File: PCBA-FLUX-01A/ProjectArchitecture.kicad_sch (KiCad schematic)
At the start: 0 parts

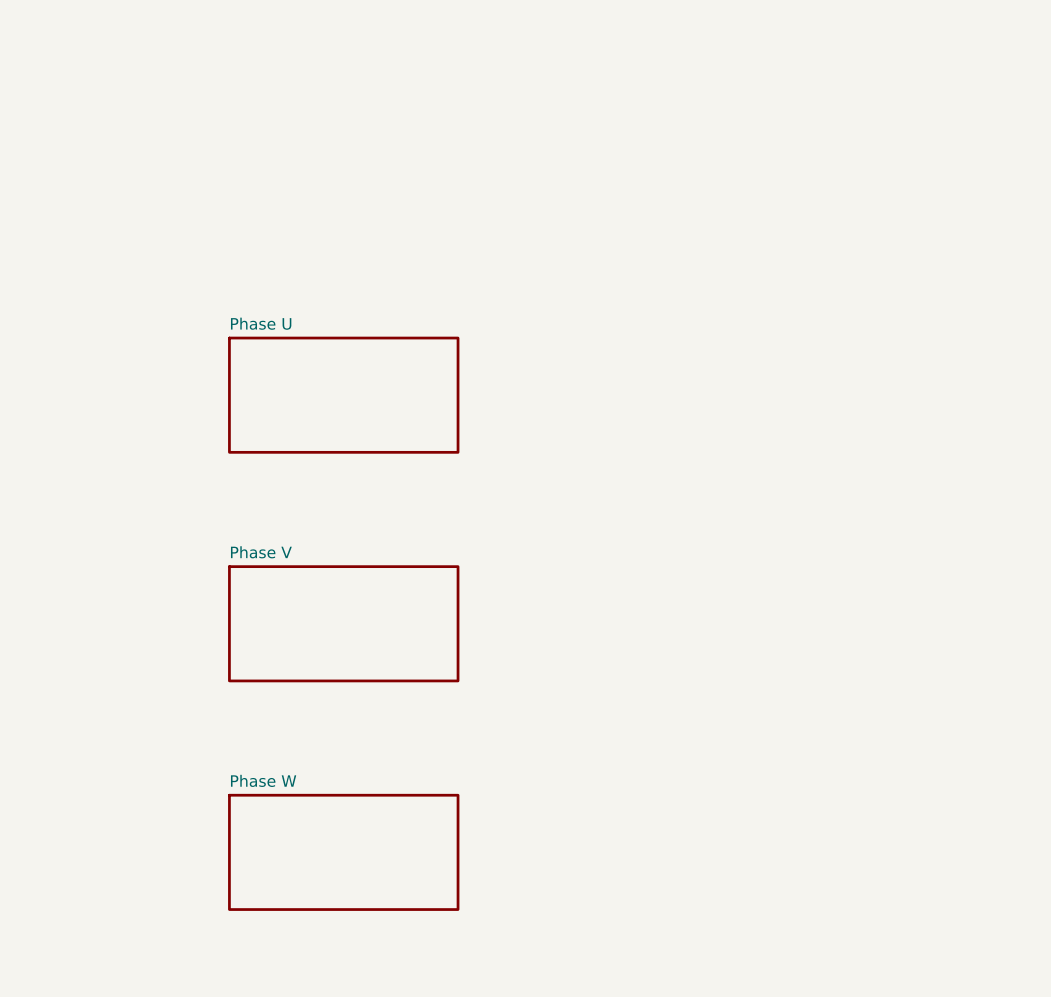
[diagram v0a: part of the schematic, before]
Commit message: Changes were made
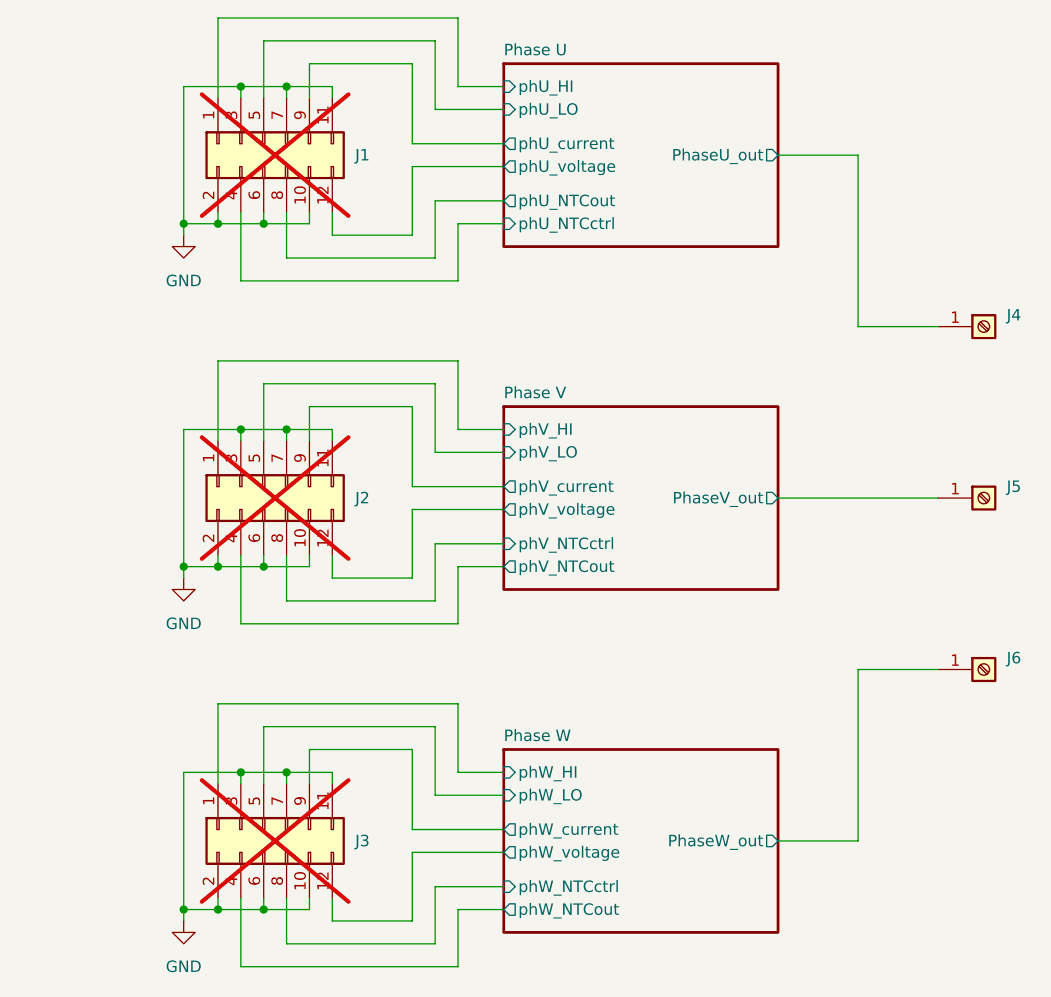
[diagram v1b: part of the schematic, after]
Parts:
- added J1, J2, J3: Conn_02x06_Odd_Even, Connector_PinHeader_2.54mm:PinHeader_2x06_P2.54mm_Vertical, symbol Connector_Generic:Conn_02x06_Odd_Even
- added J4, J5, J6: Screw_Terminal_01x01, symbol Connector:Screw_Terminal_01x01
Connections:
- new net GND: J1.10 (Pin_10), J1.11 (Pin_11), J1.2 (Pin_2), J1.3 (Pin_3), J1.6 (Pin_6), J1.7 (Pin_7), J2.10 (Pin_10), J2.11 (Pin_11), J2.2 (Pin_2), J2.3 (Pin_3), J2.6 (Pin_6), J2.7 (Pin_7), J3.10 (Pin_10), J3.11 (Pin_11), J3.2 (Pin_2), J3.3 (Pin_3), J3.6 (Pin_6), J3.7 (Pin_7)
- new net Phase U/PhaseU_out: J4.1 (Pin_1)
- new net Phase U/phU_HI: J1.1 (Pin_1)
- new net Phase U/phU_LO: J1.5 (Pin_5)
- new net Phase U/phU_NTCctrl: J1.4 (Pin_4)
- new net Phase U/phU_NTCout: J1.8 (Pin_8)
- new net Phase U/phU_current: J1.9 (Pin_9)
- new net Phase U/phU_voltage: J1.12 (Pin_12)
- new net Phase V/PhaseV_out: J5.1 (Pin_1)
- new net Phase V/phV_HI: J2.1 (Pin_1)
- new net Phase V/phV_LO: J2.5 (Pin_5)
- new net Phase V/phV_NTCctrl: J2.8 (Pin_8)
- new net Phase V/phV_NTCout: J2.4 (Pin_4)
- new net Phase V/phV_current: J2.9 (Pin_9)
- new net Phase V/phV_voltage: J2.12 (Pin_12)
- new net Phase W/PhaseW_out: J6.1 (Pin_1)
- new net Phase W/phW_HI: J3.1 (Pin_1)
- new net Phase W/phW_LO: J3.5 (Pin_5)
- new net Phase W/phW_NTCctrl: J3.8 (Pin_8)
- new net Phase W/phW_NTCout: J3.4 (Pin_4)
- new net Phase W/phW_current: J3.9 (Pin_9)
- new net Phase W/phW_voltage: J3.12 (Pin_12)
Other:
- sheet Phase U ports: added PhaseU_out, phU_HI, phU_LO, phU_NTCctrl, phU_NTCout, phU_current, phU_voltage; removed none
- sheet Phase V ports: added PhaseV_out, phV_HI, phV_LO, phV_NTCctrl, phV_NTCout, phV_current, phV_voltage; removed none
- sheet Phase W ports: added PhaseW_out, phW_HI, phW_LO, phW_NTCctrl, phW_NTCout, phW_current, phW_voltage; removed none

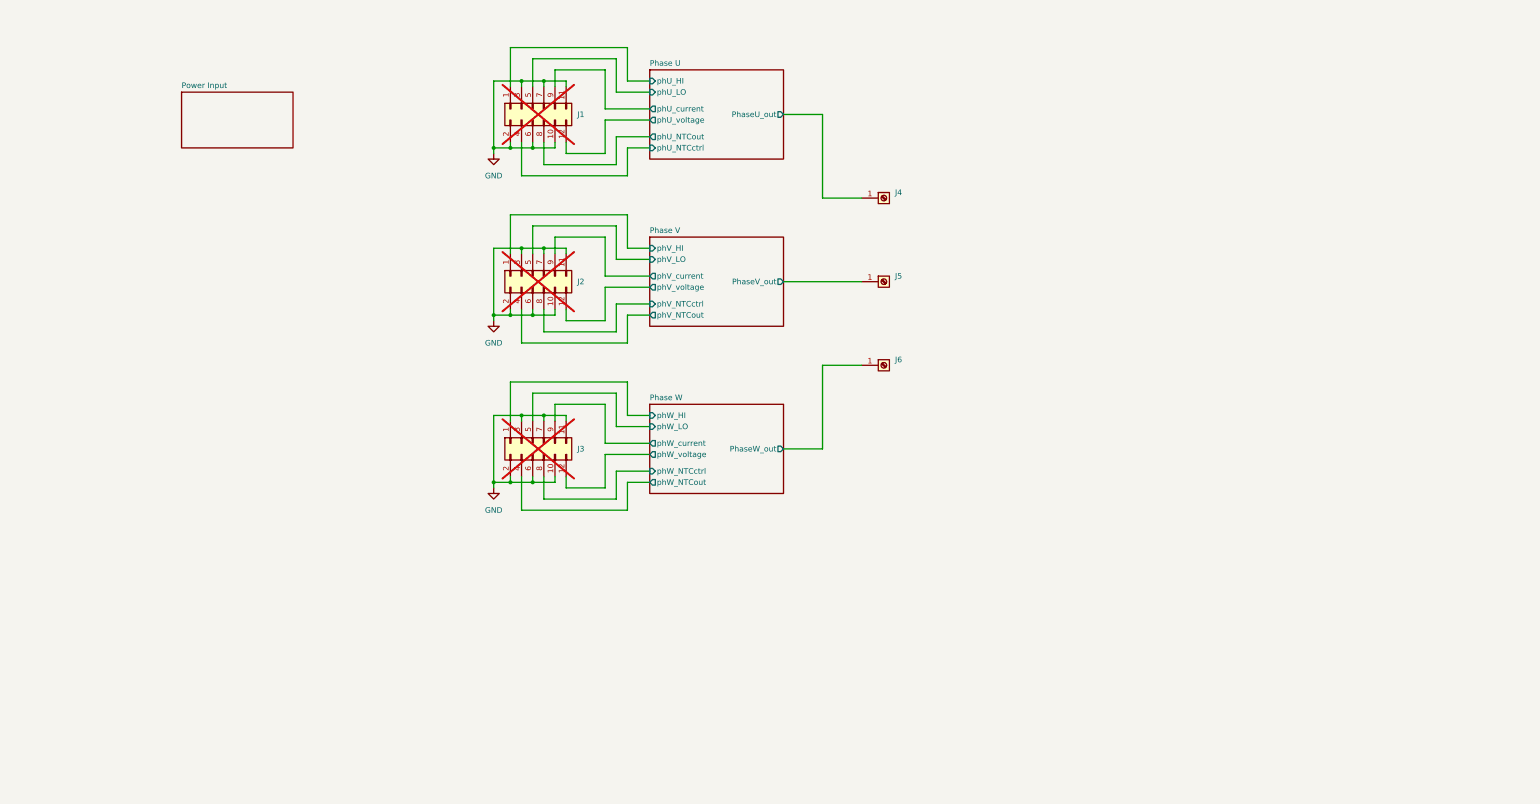
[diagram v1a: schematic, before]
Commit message: Finished schematic?
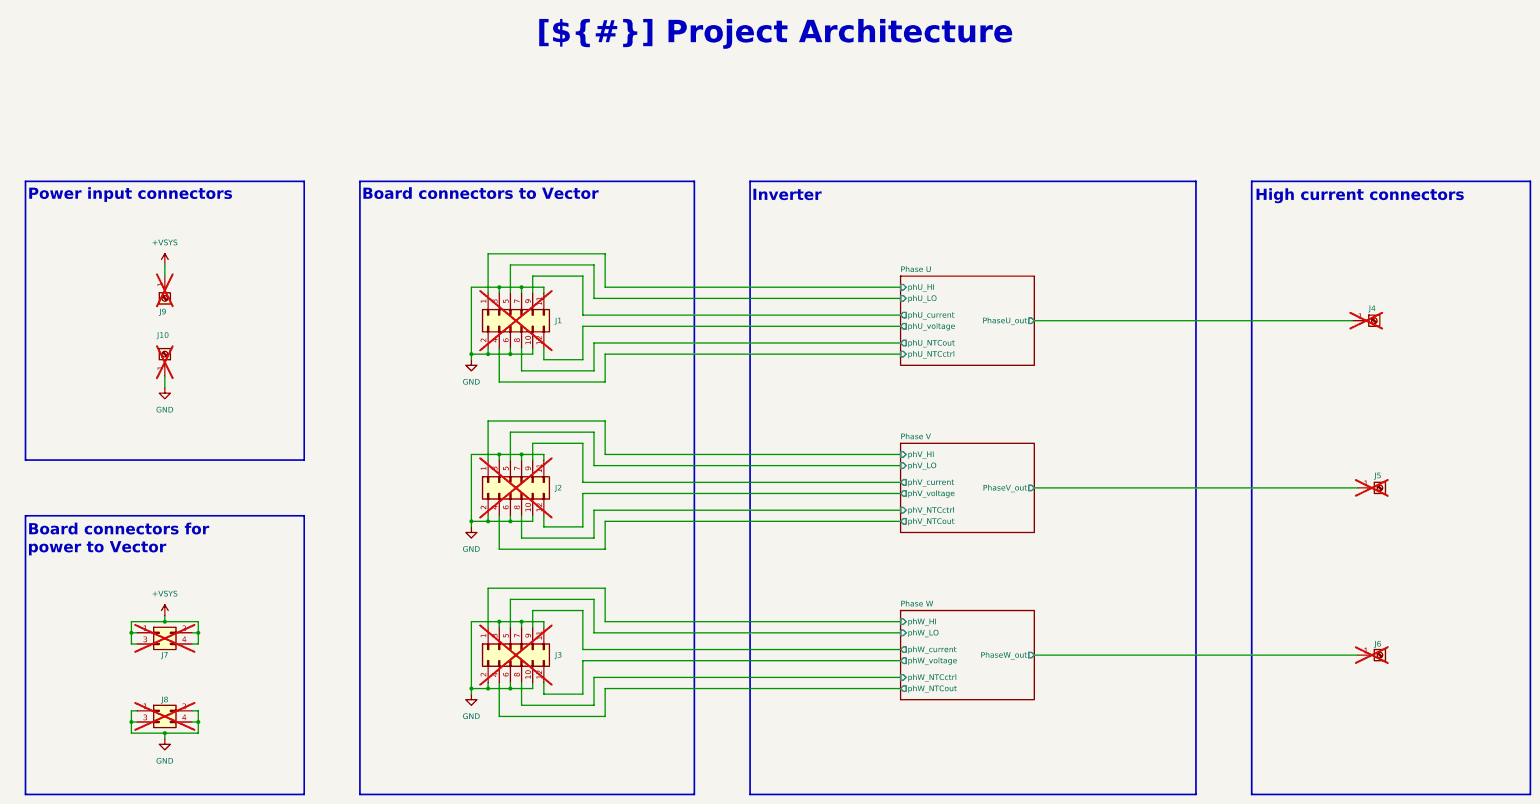
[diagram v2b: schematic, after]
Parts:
- added J10, J9: Screw_Terminal_01x01, Bvrny's_library:M8_NutTerminal, symbol Connector:Screw_Terminal_01x01
- added J7, J8: Conn_02x02_Odd_Even, Connector_PinHeader_2.54mm:PinHeader_2x02_P2.54mm_Vertical, symbol Connector_Generic:Conn_02x02_Odd_Even
- J4, J5, J6: footprint (none) -> Bvrny's_library:M8_NutTerminal; now not fitted
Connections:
- net GND: now also J10.1 (Pin_1), J8.1 (Pin_1), J8.2 (Pin_2), J8.3 (Pin_3), J8.4 (Pin_4)
- new net +VSYS: J7.1 (Pin_1), J7.2 (Pin_2), J7.3 (Pin_3), J7.4 (Pin_4), J9.1 (Pin_1)
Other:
- removed sheet Power Input
- note added: "Board connectors for power to Vector"
- note added: "Board connectors to Vector"
- note added: "High current connectors"
- note added: "Inverter"
- note added: "Power input connectors"
- moved on the sheet: J1, J2, J3
